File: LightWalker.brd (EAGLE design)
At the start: 78 x 76 mm, 35 parts, among them IC1 74HCT245N

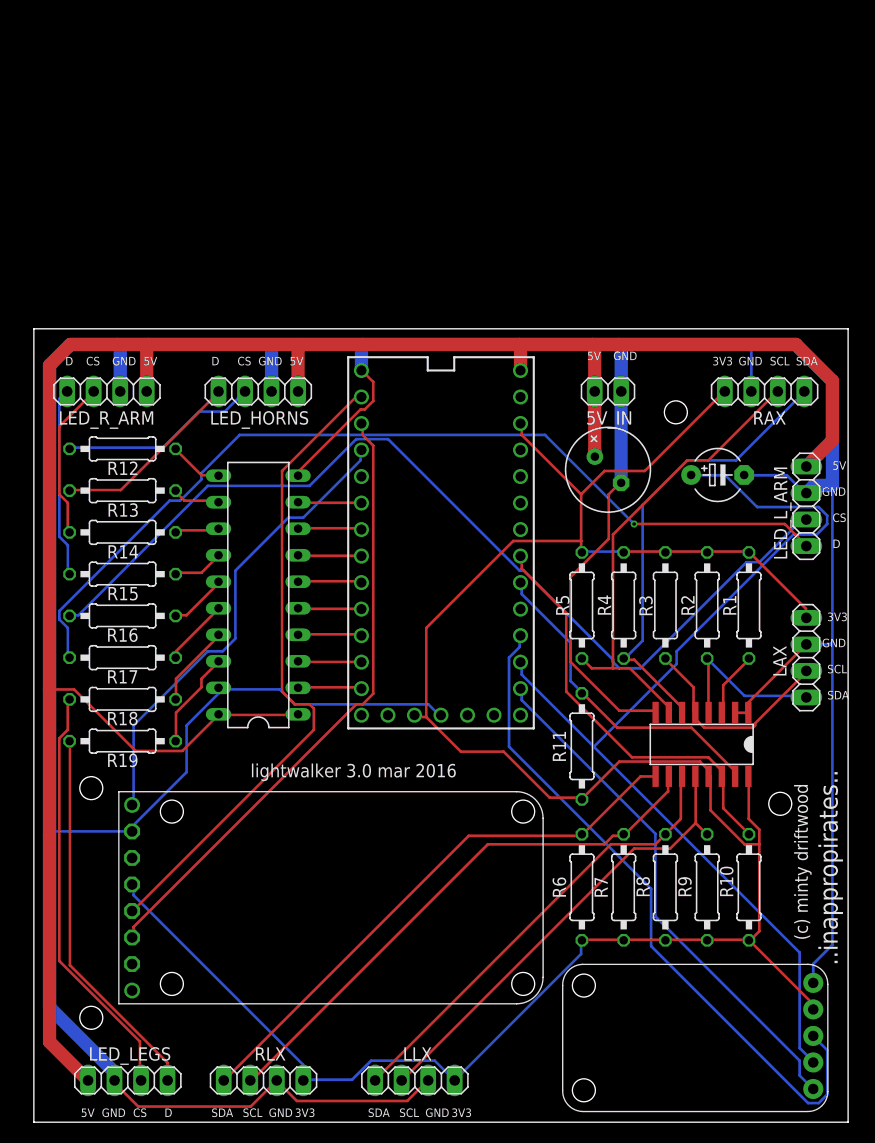
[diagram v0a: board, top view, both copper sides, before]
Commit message: lightwalker PCB 4.0
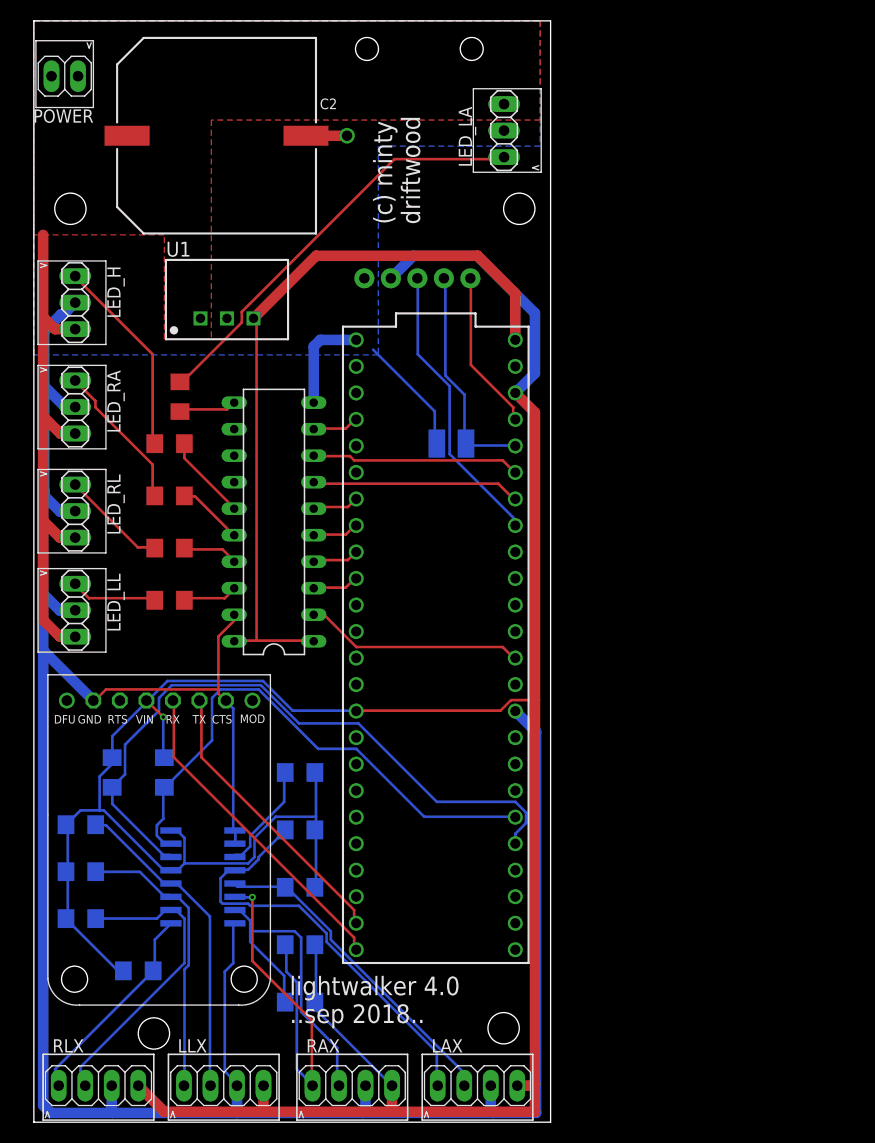
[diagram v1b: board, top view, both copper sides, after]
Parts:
- removed 5V_IN: (no value), pinhead:1X02
- removed BLUEFRUIT1: BLUEFRUIT_EZLINK, minty:BLUEFRUIT
- removed BRAINS: TEENSY_3.0_BASIC, Teensy3.0:TEENSY_3.0_BASIC
- removed C4: 0.1uf, rcl:E5-5
- removed LED_HORNS, LED_LEGS, LED_L_ARM, LED_R_ARM: (no value), pinhead:1X04
- removed MAX9814MIC: MAX9814MIC, minty:MAX9814MIC
- removed R17, R18, R19: 100, resistor:0207/10
- added BRAIN: TEENSY_3.6_DIL, Teensy3.0:TEENSY_3.6_DIL
- added C3: 0.1uf, cap-master.rpt:3225
- added LED_H, LED_LA, LED_LL, LED_RA, LED_RL: 2.54MM_TERMINAL_BLOCK-3, minty:TB_1X3
- added POWER: 2.54MM_TERMINAL_BLOCK-2, minty:TB_1X2
- added U$1: BLUEFRUIT_BLE_UART_FRIENDALL, minty:BLUEFRUIT_BLE_UART_FRIEND_ALL
- added U$4: MAX9814MICALL, minty:MAX9814MIC
- added U1: TSR_1-2450, _traco_tsr-1:TSR-1
- C2: device rcl:E3,5-8 -> cap-master:SV-K
- LAX, LLX, RAX, RLX: value (none) -> 2.54MM_TERMINAL_BLOCK-4; device pinhead:1X04 -> minty:TB_1X4
- R1, R10, R11, R12, R13, R14, R15, R16, R2, R3, R4, R5, R6, R7, R8, R9: device resistor:0207/10 -> resistor:R1206
- moved RAX 77.3 mm to (30.5, 3.60)
- moved R10 62.0 mm to (7.50, 33.5), flipped to the bottom, turned to 270 degrees
- moved R9 60.3 mm to (4.50, 28.5), flipped to the bottom, turned to 180 degrees
- moved R8 56.0 mm to (4.50, 24.0), flipped to the bottom, turned to 180 degrees
- moved R7 52.1 mm to (4.50, 19.5), flipped to the bottom, turned to 180 degrees
- moved LAX 51.6 mm to (42.5, 3.60), turned to 0 degrees
- moved I2CMULTI1 49.6 mm to (16.0, 23.5), flipped to the bottom, turned to 270 degrees
- moved C2 49.3 mm to (17.5, 94.5), turned to 0 degrees
- moved R5 46.6 mm to (25.5, 11.5), flipped to the bottom, turned to 0 degrees
- moved R1 45.9 mm to (25.5, 33.5), flipped to the bottom, turned to 0 degrees
- moved R4 44.9 mm to (25.5, 17.0), flipped to the bottom, turned to 0 degrees
- moved R2 44.5 mm to (25.5, 28.0), flipped to the bottom, turned to 0 degrees
- moved R3 44.2 mm to (25.5, 22.5), flipped to the bottom, turned to 0 degrees
- moved R6 43.2 mm to (10.0, 14.5), flipped to the bottom, turned to 180 degrees
- moved R11 40.1 mm to (12.5, 33.5), flipped to the bottom, turned to 270 degrees
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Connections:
- removed net 3V: BLUEFRUIT1.3V
- removed net BT_STATUS: BLUEFRUIT1.STS, BRAINS.2
- removed net CS0: LED_HORNS.2, R12.1
- removed net CS1: LED_R_ARM.2, R14.1
- removed net CS2: LED_L_ARM.2, R16.1
- removed net CS3: LED_LEGS.2, R18.1
- removed net DATA0: LED_HORNS.1, R13.1
- removed net DATA1: LED_R_ARM.1, R15.1
- removed net DATA2: LED_L_ARM.1, R17.1
- removed net DATA3: LED_LEGS.1, R19.1
- removed net N$14: BRAINS.7, IC1.6
- removed net N$15: BRAINS.8, IC1.5
- removed net N$16: BRAINS.9, IC1.4
- removed net N$17: BRAINS.10, IC1.3
- removed net N$18: BRAINS.11, IC1.2
- removed net N$4: IC1.13, R14.2
- removed net N$7: IC1.16, R17.2
- removed net N$8: IC1.17, R18.2
- removed net N$9 (its old number): IC1.18, R19.2
- removed net VBAT: BRAINS.VBAT
- new net 12V: C2.+, LED_H.3, LED_LA.3, LED_LL.3, LED_RA.3, LED_RL.3, POWER.2, U1.1
- new net 20: BRAIN.20/A6, IC1.7
- new net 21: BRAIN.21/A7, IC1.8
- new net LED_DATA_0: LED_LA.1, R12.1
- new net LED_DATA_1: LED_LL.1, R16.1
- new net LED_DATA_2: LED_RL.1, R14.1
- new net LED_DATA_3: LED_RA.1, R15.1
- new net LED_DATA_4: LED_H.1, R13.1
- new net N$1: BRAIN.2, IC1.9
- new net N$12: IC1.17, R15.2
- new net N$2: BRAIN.5, IC1.6
- new net PIN14: BRAIN.14/A0, IC1.2
- net +3V3: now also BRAIN.3.3V, BRAIN.3.3V3, LAX.4, LLX.4, RAX.4, RLX.4, U$1.VIN, U$4.VDD; no longer BLUEFRUIT1.VIN, BRAINS.3.3V, BRAINS.3.3V1, LAX.1, LLX.1, MAX9814MIC.VDD, RAX.1, RLX.1
- net +5V: now also BRAIN.VIN, U1.3; no longer 5V_IN.1, BRAINS.VIN, C2.+, LED_HORNS.4, LED_LEGS.4, LED_L_ARM.4, LED_R_ARM.4
- net AGND: now also BRAIN.AGND; no longer BRAINS.AGND
- net AR: now also BRAIN.23/A9, U$4.AR; no longer BRAINS.14/A0, MAX9814MIC.AR
- net GAIN: now also BRAIN.19/A5, U$4.GAIN; no longer BRAINS.16/A2, MAX9814MIC.GAIN
- net GND: now also BRAIN.GND, BRAIN.GND1, C3.2, LAX.3, LED_H.2, LED_LA.2, LED_LL.2, LED_RA.2, LED_RL.2, LLX.3, POWER.1, RAX.3, RLX.3, U$1.CTS, U$1.GND, U$4.GND, U1.2; no longer 5V_IN.2, BLUEFRUIT1.GND, BRAINS.GND, BRAINS.GND1, C4.-, LAX.2, LED_HORNS.3, LED_LEGS.3, LED_L_ARM.3, LED_R_ARM.3, LLX.2, MAX9814MIC.GND, RAX.2, RLX.2
- net MIC_OUT: now also BRAIN.22/A8, C3.1, U$4.OUT; no longer BRAINS.15/A1, C4.+, MAX9814MIC.OUT
- net N$10: now also IC1.15, R13.2; no longer BRAINS.4, IC1.9
- net N$11: now also IC1.16, R14.2; no longer BRAINS.5, IC1.8
- net N$13: now also IC1.18, R16.2; no longer BRAINS.6, IC1.7
- net N$3: now also BRAIN.6, IC1.5; no longer IC1.12, R13.2
- net N$5: now also BRAIN.7, IC1.4; no longer IC1.14, R15.2
- net N$6: now also BRAIN.8, IC1.3; no longer IC1.15, R16.2
- net RX: now also BRAIN.31/A12, U$1.TX0; no longer BLUEFRUIT1.TX, BRAINS.0
- net SCL: now also BRAIN.37/A18; no longer BRAINS.19/A5
- net SCL0: now also LAX.2; no longer LAX.3
- net SCL1: now also RAX.2; no longer RAX.3
- net SCL2: now also RLX.2; no longer RLX.3
- net SCL3: now also LLX.2; no longer LLX.3
- net SDA: now also BRAIN.38/A19; no longer BRAINS.18/A4
- net SDA0: now also LAX.1; no longer LAX.4
- net SDA1: now also RAX.1; no longer RAX.4
- net SDA2: now also RLX.1; no longer RLX.4
- net SDA3: now also LLX.1; no longer LLX.4
- net TX: now also BRAIN.32/A13, U$1.RXI; no longer BLUEFRUIT1.RX, BRAINS.1
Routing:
- net +5V: track 206.8 -> 72.1 mm
- net GND: track 384.8 -> 271.6 mm, vias 0 -> 1
- net CS2: track 92.7 -> 0.00 mm
- net DATA2: track 88.3 -> 0.00 mm, vias 1 -> 0
- net MIC_OUT: track 97.3 -> 21.6 mm
- net 12V: track 0.00 -> 51.7 mm
- net +3V3: track 229.9 -> 278.2 mm, vias 0 -> 1
- net BT_STATUS: track 44.8 -> 0.00 mm
- net LED_DATA_0: track 0.00 -> 40.7 mm
- net CS3: track 40.2 -> 0.00 mm
- net GAIN: track 65.4 -> 27.6 mm
- net DATA3: track 36.4 -> 0.00 mm
- net AR: track 50.0 -> 15.3 mm
- net RX: track 62.1 -> 27.6 mm
- net SDA2: track 53.4 -> 20.3 mm
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- added copper zone on layer 1, net 12V
- added copper zone on layer 16, net GND
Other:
- board size 78 x 76 mm -> 49.5 x 105.5 mm
- board text added: ".. inappropirates .."
- board text added: "lightwalker 4.0 ..sep 2018.."
- board text removed: "..inappropirates.."
- board text removed: "3V3"
- board text removed: "5V"
- board text removed: "CS"
- board text removed: "D"
- board text removed: "GND"
- board text removed: "SCL"
- board text removed: "SDA"
- board text removed: "lightwalker 3.0 mar 2016"
